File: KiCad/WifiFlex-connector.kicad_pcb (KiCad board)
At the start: 2 copper layers, 28.8 x 10.5 mm, 1 part, among them J1 Conn_01x20_Pin

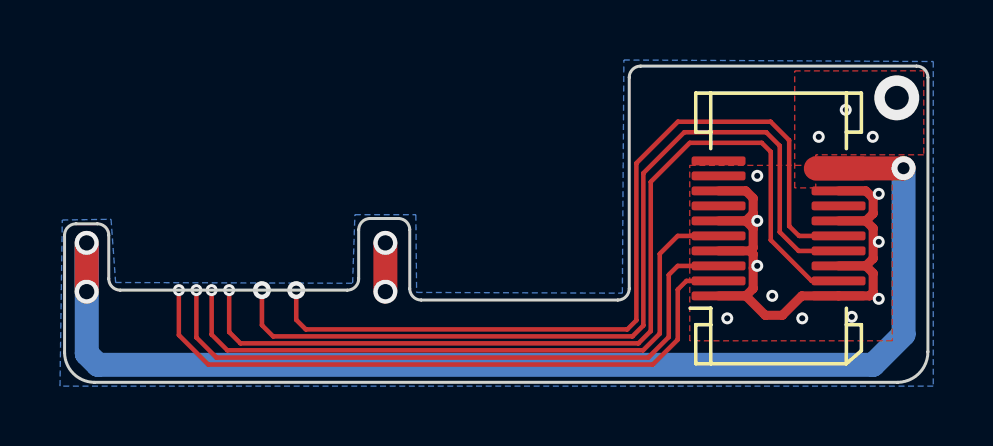
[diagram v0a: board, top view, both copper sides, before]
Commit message: add modified files
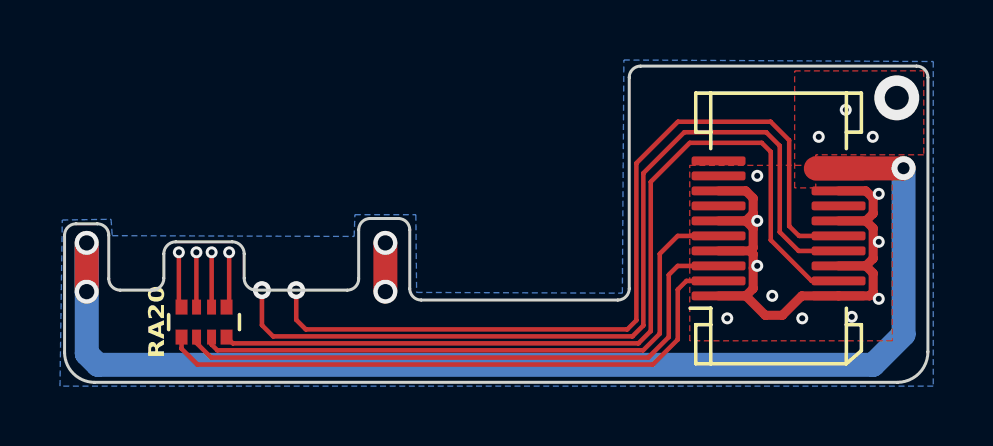
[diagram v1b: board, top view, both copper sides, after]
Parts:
- added RA20: R_Pack04, Resistor_SMD:R_Array_Convex_4x0402, F.Cu at (159.3, 77.9)
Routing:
- net Net-(J2-Pin_6): track 0.00 -> 1.86 mm, vias 0 -> 1
- net Net-(J2-Pin_3): track 0.00 -> 1.86 mm, vias 0 -> 1
- net Net-(J2-Pin_5): track 0.00 -> 1.83 mm, vias 0 -> 1
- net Net-(J2-Pin_4): track 0.00 -> 1.83 mm, vias 0 -> 1
- net Net-(J1-Pin_3): track 21.7 -> 20.3 mm, vias 1 -> 0
- net Net-(J1-Pin_2): track 22.0 -> 20.6 mm, vias 1 -> 0
- net Net-(J1-Pin_19): track 31.2 -> 29.8 mm, vias 1 -> 0
- net Net-(J1-Pin_5): track 22.7 -> 21.3 mm, vias 1 -> 0
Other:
- outline, holes or cut-outs redrawn
